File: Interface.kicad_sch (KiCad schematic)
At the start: 12 parts, among them J2 Conn_01x02_Pin, J3 Conn_01x02_Pin, U8 TCAN1042HGVDRBRQ1

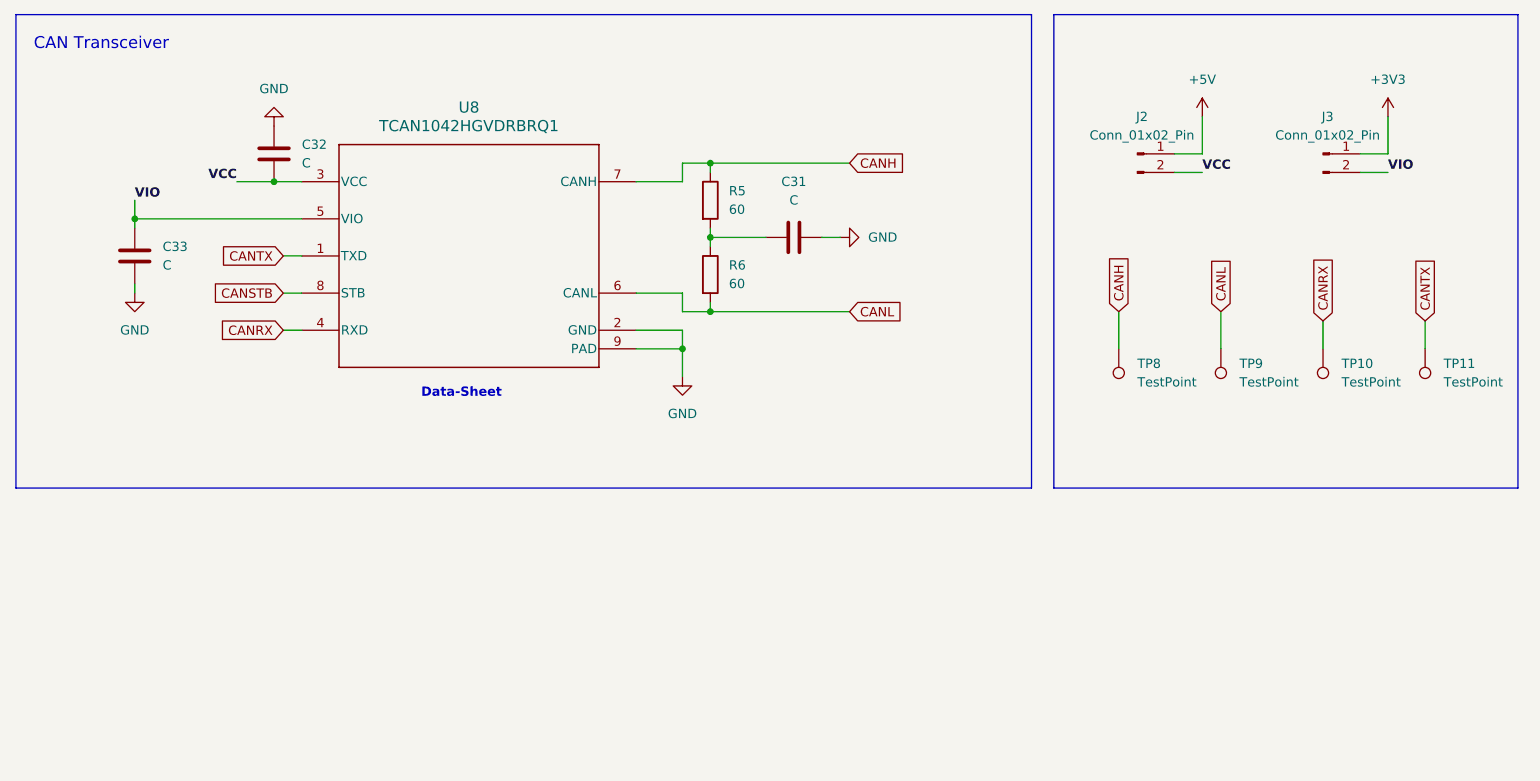
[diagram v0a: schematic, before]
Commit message: #
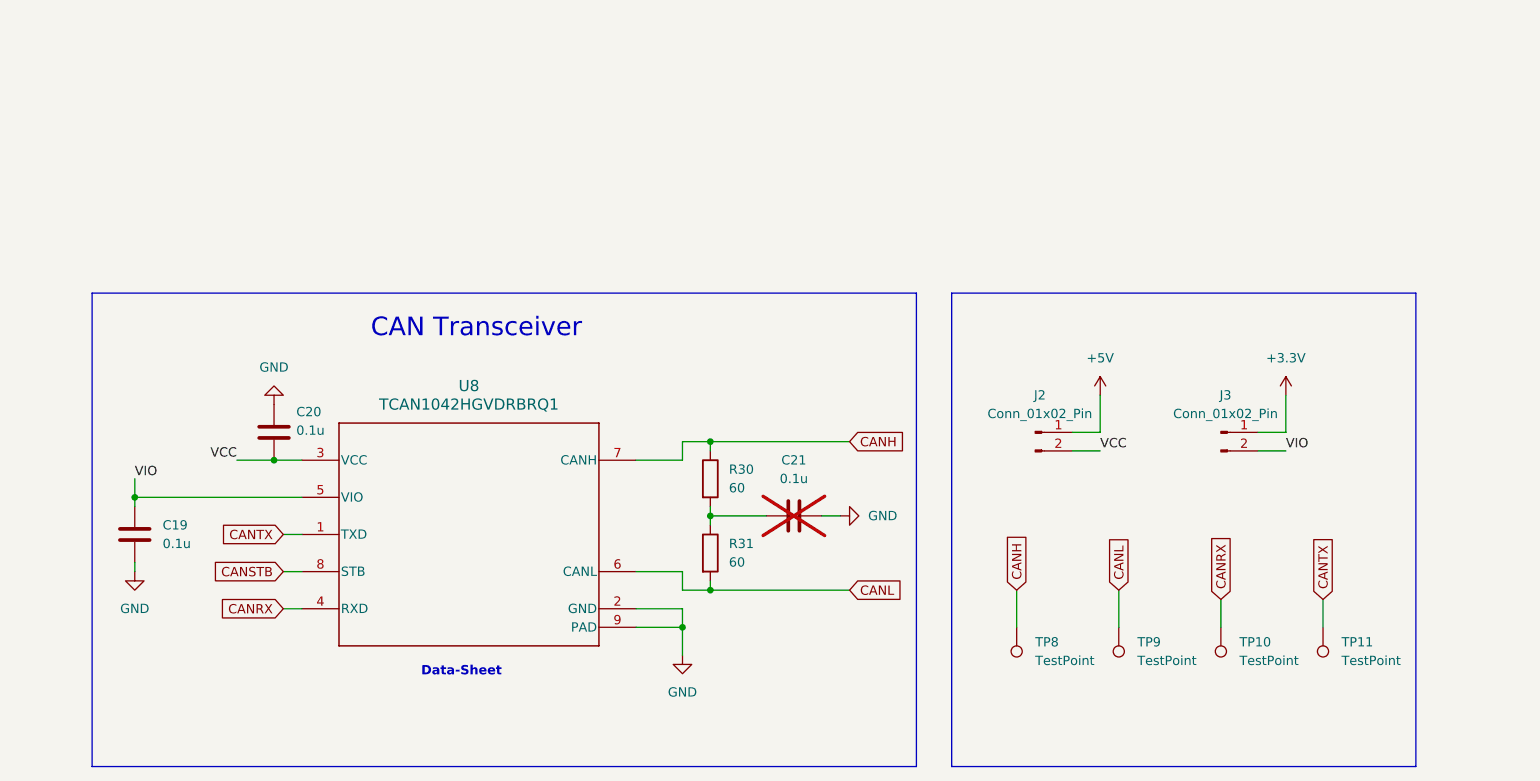
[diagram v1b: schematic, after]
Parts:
- C19: renamed from C33; value C -> 0.1u
- C20: renamed from C32; value C -> 0.1u
- C21: renamed from C31; value C -> 0.1u; now not fitted
- U8: footprint DRB0008F -> Footprint:DRB0008F
- renumbered R5 to R30, R6 to R31
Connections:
- net +3V3 renamed +3.3V
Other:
- moved on the sheet: C19, C20, J2, J3, R30, R31, TP10, TP11, TP8, TP9, U8
